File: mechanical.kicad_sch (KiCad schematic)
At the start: 16 parts

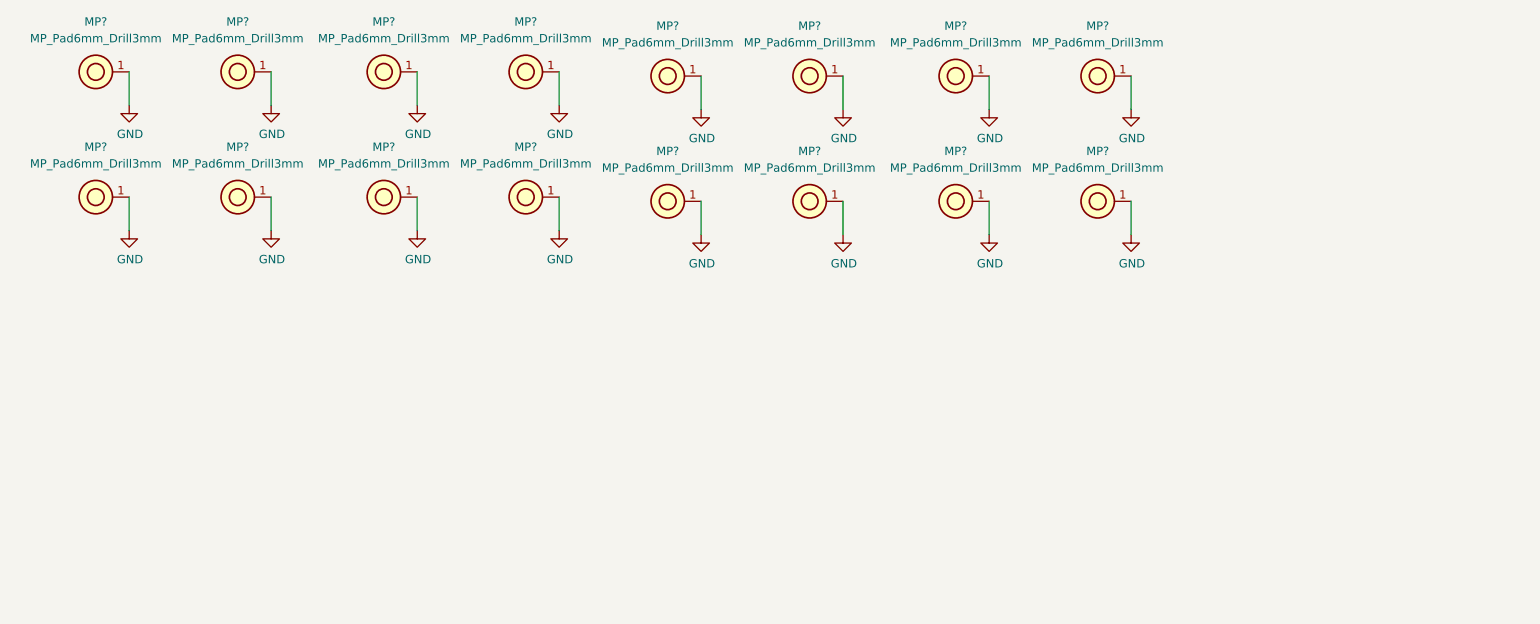
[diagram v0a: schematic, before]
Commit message: Cosmetic changes
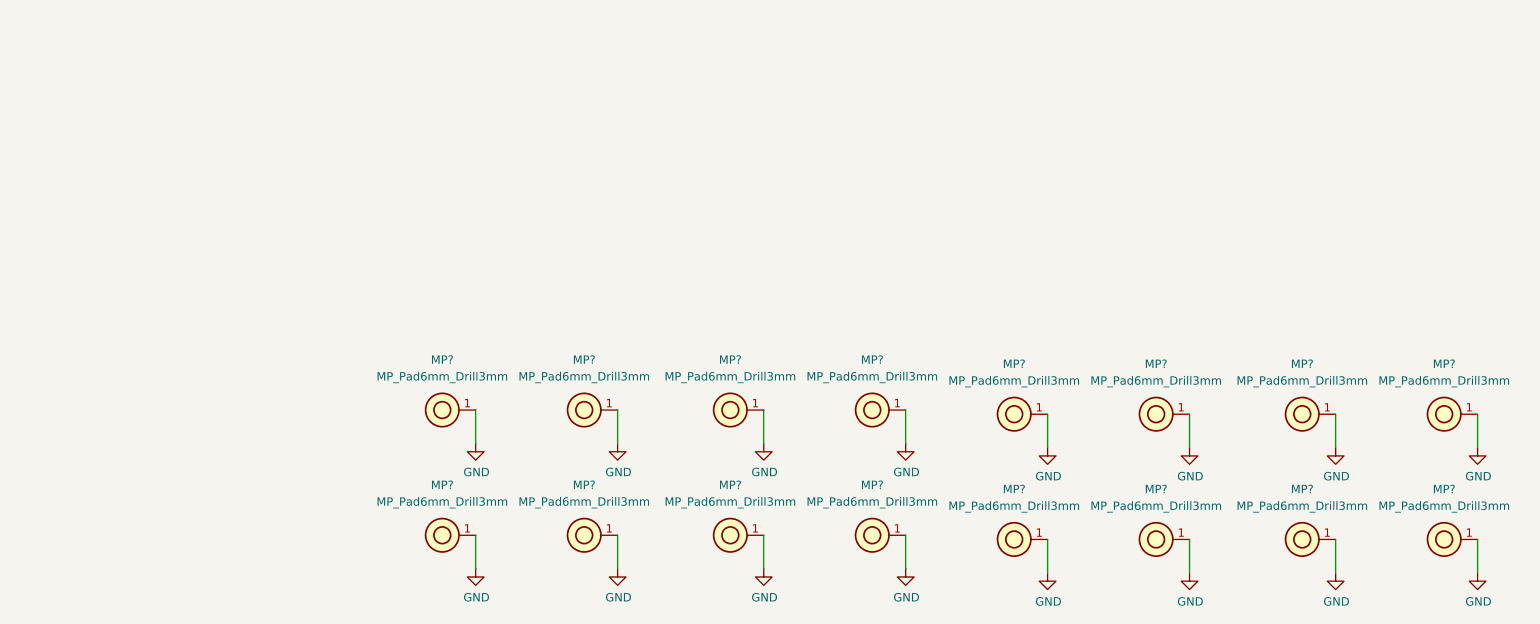
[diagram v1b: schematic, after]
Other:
- moved on the sheet: MP?
